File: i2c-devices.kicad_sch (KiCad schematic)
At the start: 7 parts, among them IC17 AT24CS01-ST

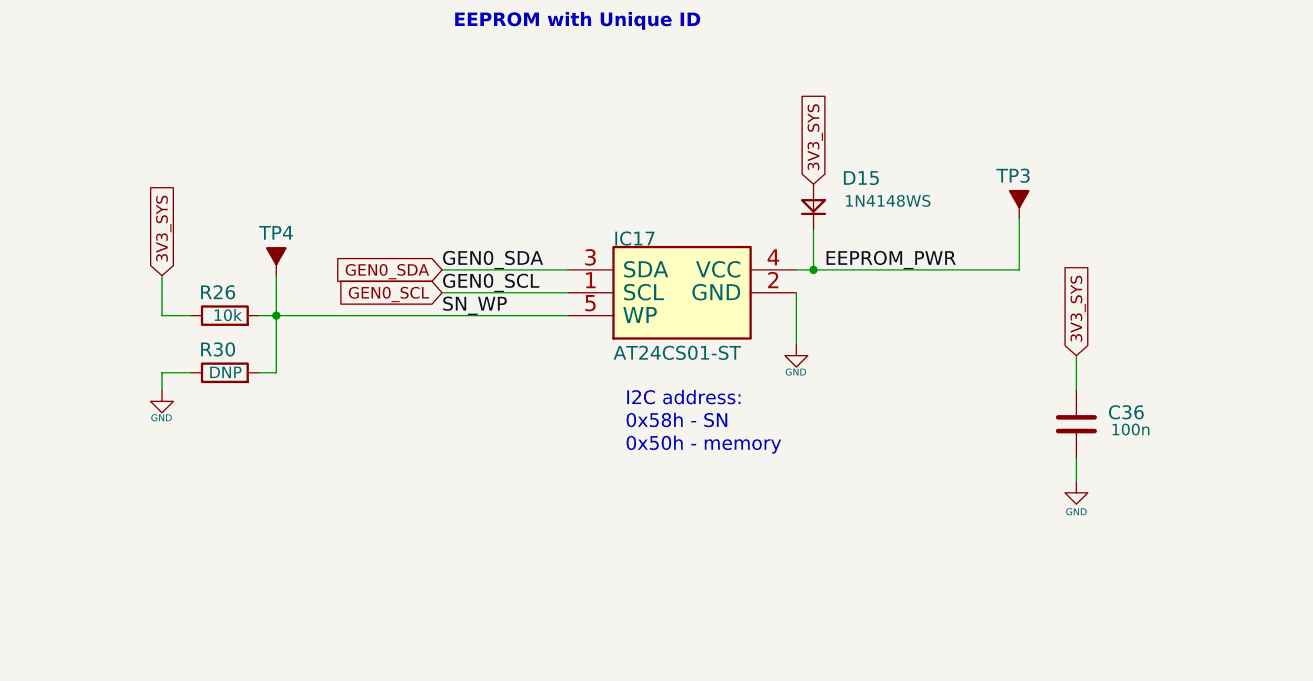
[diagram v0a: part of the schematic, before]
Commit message: Checkpoint
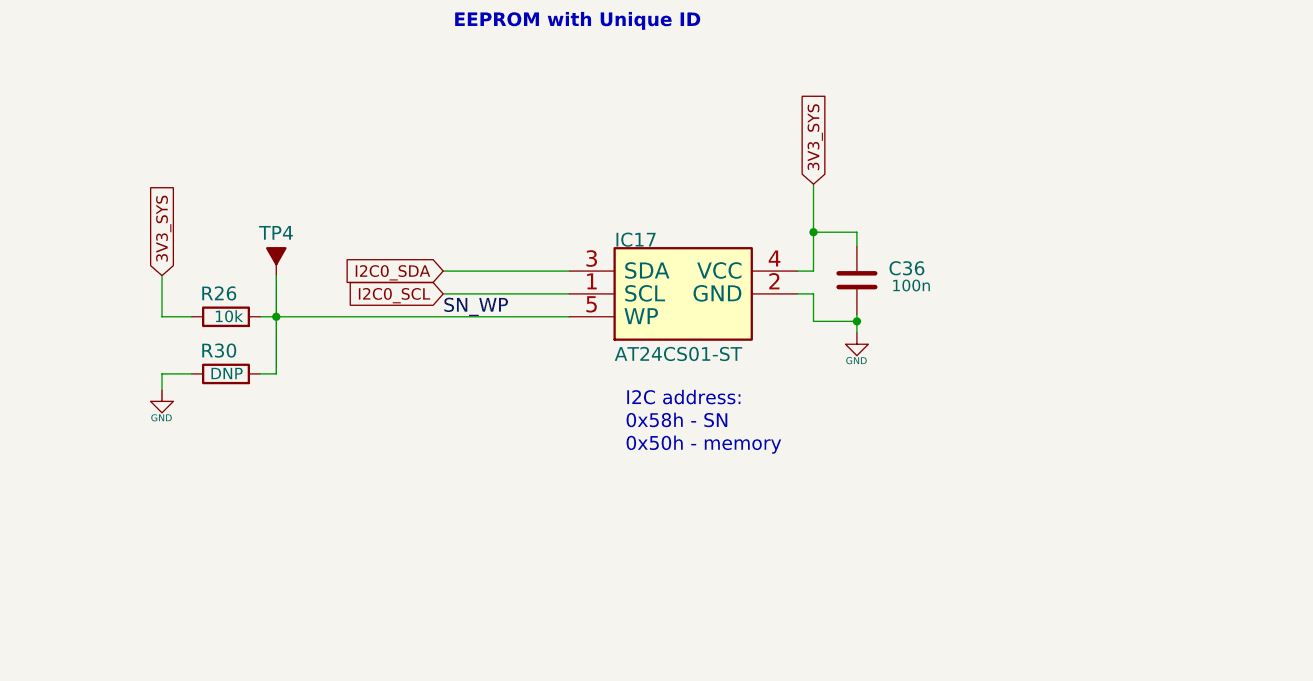
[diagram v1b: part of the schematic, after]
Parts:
- removed D15: diode, jetson-nano-baseboard-footprints:SOD-323, symbol jetson-nano-baseboard:diode
- removed TP3: Testpad, jetson-nano-baseboard-footprints:TP-R-1.5, symbol jetson-nano-baseboard:Testpad
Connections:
- net EEPROM_PWR is gone; now on net 3V3_SYS: IC17.4 (VCC)
- net GEN0_SCL renamed I2C0_SCL
- net GEN0_SDA renamed I2C0_SDA
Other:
- moved on the sheet: C36
